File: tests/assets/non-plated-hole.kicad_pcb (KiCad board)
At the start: 2 copper layers, 50 x 50 mm, 2 parts

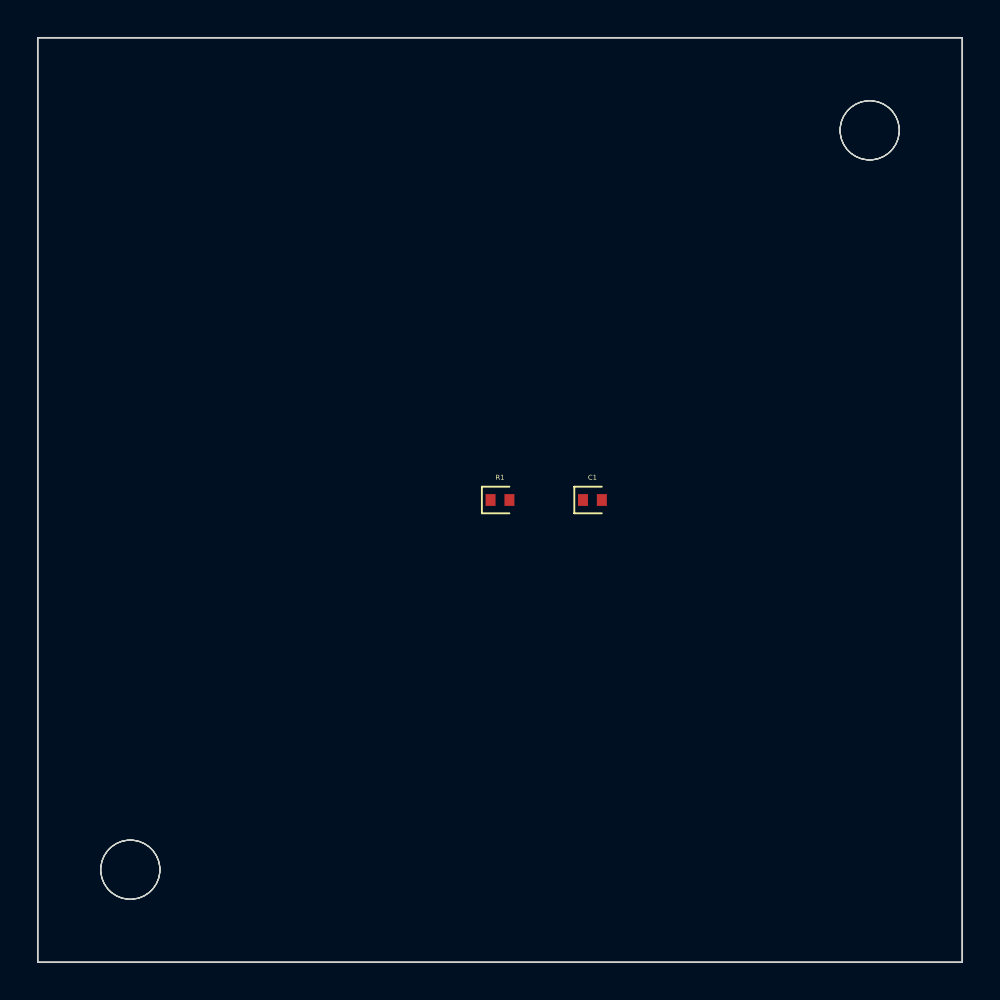
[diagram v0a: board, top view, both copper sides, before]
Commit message: up
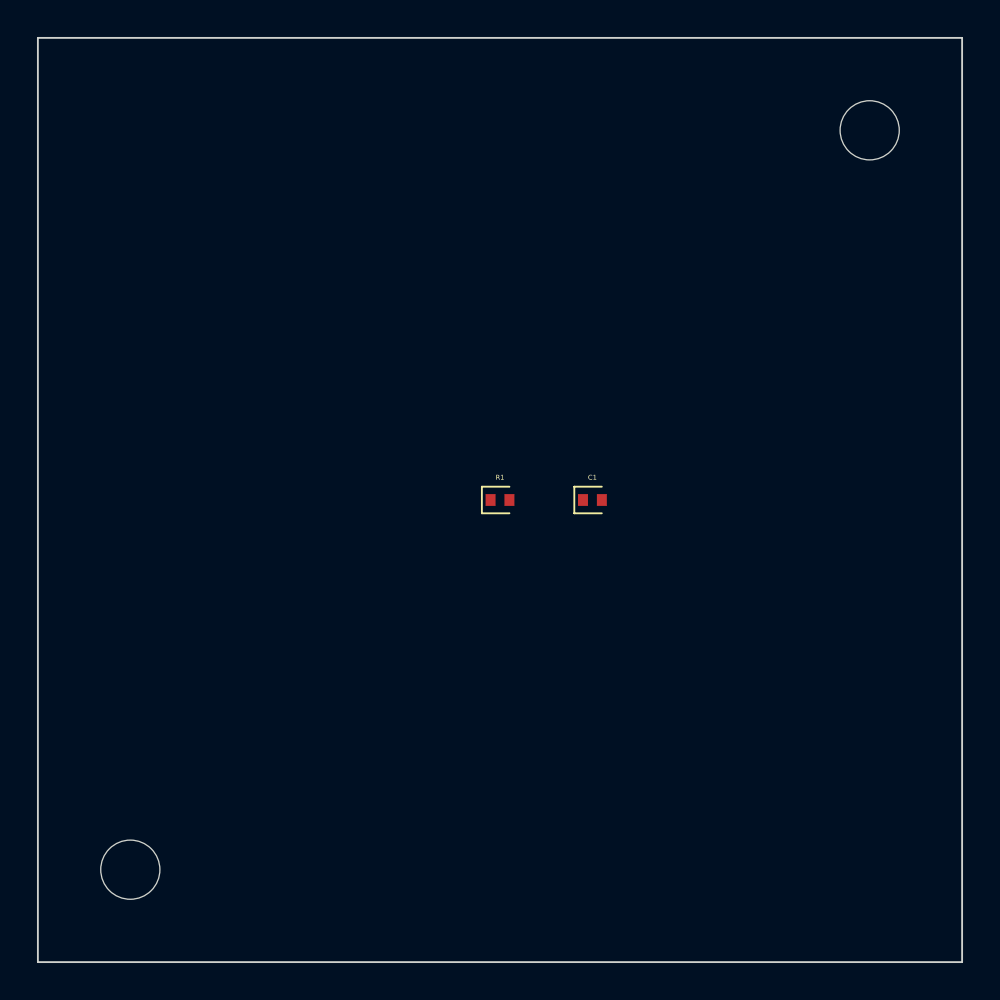
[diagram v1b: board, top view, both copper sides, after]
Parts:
- added ?: , tscircuit:mounting_hole, F.Cu at (80.0, 120.0)
- added ?: , tscircuit:mounting_hole, F.Cu at (120.0, 80.0)
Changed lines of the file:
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@@
       )
-    )
-    (fp_rect
-      (start -1.23 -0.97)
-      (end 1.0299999999999998 0.97)
-      (layer F.CrtYd)
-      (stroke
-        (width 0.05)
-        (type default)
-      )
-      (fill no)
     )
     (pad "1" smd rect
@@
       (size 0.54 0.64)
       (layers F.Cu F.Paste F.Mask)
-    )
-    (pad "" np_thru_hole circle
-      (at -20 20 0)
-      (size 3.2 3.2)
-      (drill 3.2)
-      (layers *.Cu *.Mask)
-    )
-    (pad "" np_thru_hole circle
-      (at 20 -20 0)
-      (size 3.2 3.2)
-      (drill 3.2)
-      (layers *.Cu *.Mask)
     )
   )
@@
       )
     )
-    (fp_rect
-      (start -1.2299999999999995 -0.97)
-      (end 1.0300000000000002 0.97)
-      (layer F.CrtYd)
-      (stroke
-        (width 0.05)
-        (type default)
-      )
-      (fill no)
-    )
     (pad "1" smd rect
       (at -0.5099999999999998 0 0)
@@
       (layers F.Cu F.Paste F.Mask)
     )
+  )
+  (footprint
+    "tscircuit:mounting_hole"
+    (layer F.Cu)
+    (at 80 120 0)
     (pad "" np_thru_hole circle
-      (at -25 20 0)
+      (at 0 0 0)
       (size 3.2 3.2)
       (drill 3.2)
       (layers *.Cu *.Mask)
     )
+  )
+  (footprint
+    "tscircuit:mounting_hole"
+    (layer F.Cu)
+    (at 120 80 0)
     (pad "" np_thru_hole circle
-      (at 15 -20 0)
+      (at 0 0 0)
       (size 3.2 3.2)
       (drill 3.2)

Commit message: update
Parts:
- ? (x2): footprint tscircuit:mounting_hole -> tscircuit:MountingHole
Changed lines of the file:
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@@
   )
   (footprint
-    "tscircuit:mounting_hole"
+    "tscircuit:MountingHole"
     (layer F.Cu)
     (at 80 120 0)
@@
   )
   (footprint
-    "tscircuit:mounting_hole"
+    "tscircuit:MountingHole"
     (layer F.Cu)
     (at 120 80 0)
